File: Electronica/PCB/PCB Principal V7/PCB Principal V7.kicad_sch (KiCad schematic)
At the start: 18 parts, among them J1 Conexion Sensores, J11 Conn_01x04_Pin, J2 Power Monster, J3 On/Off General, J4 Power Input 2, J5 IDC Placa Botones, J6 Power Input 1, SW1 On/Off Motores, U1 74HC595

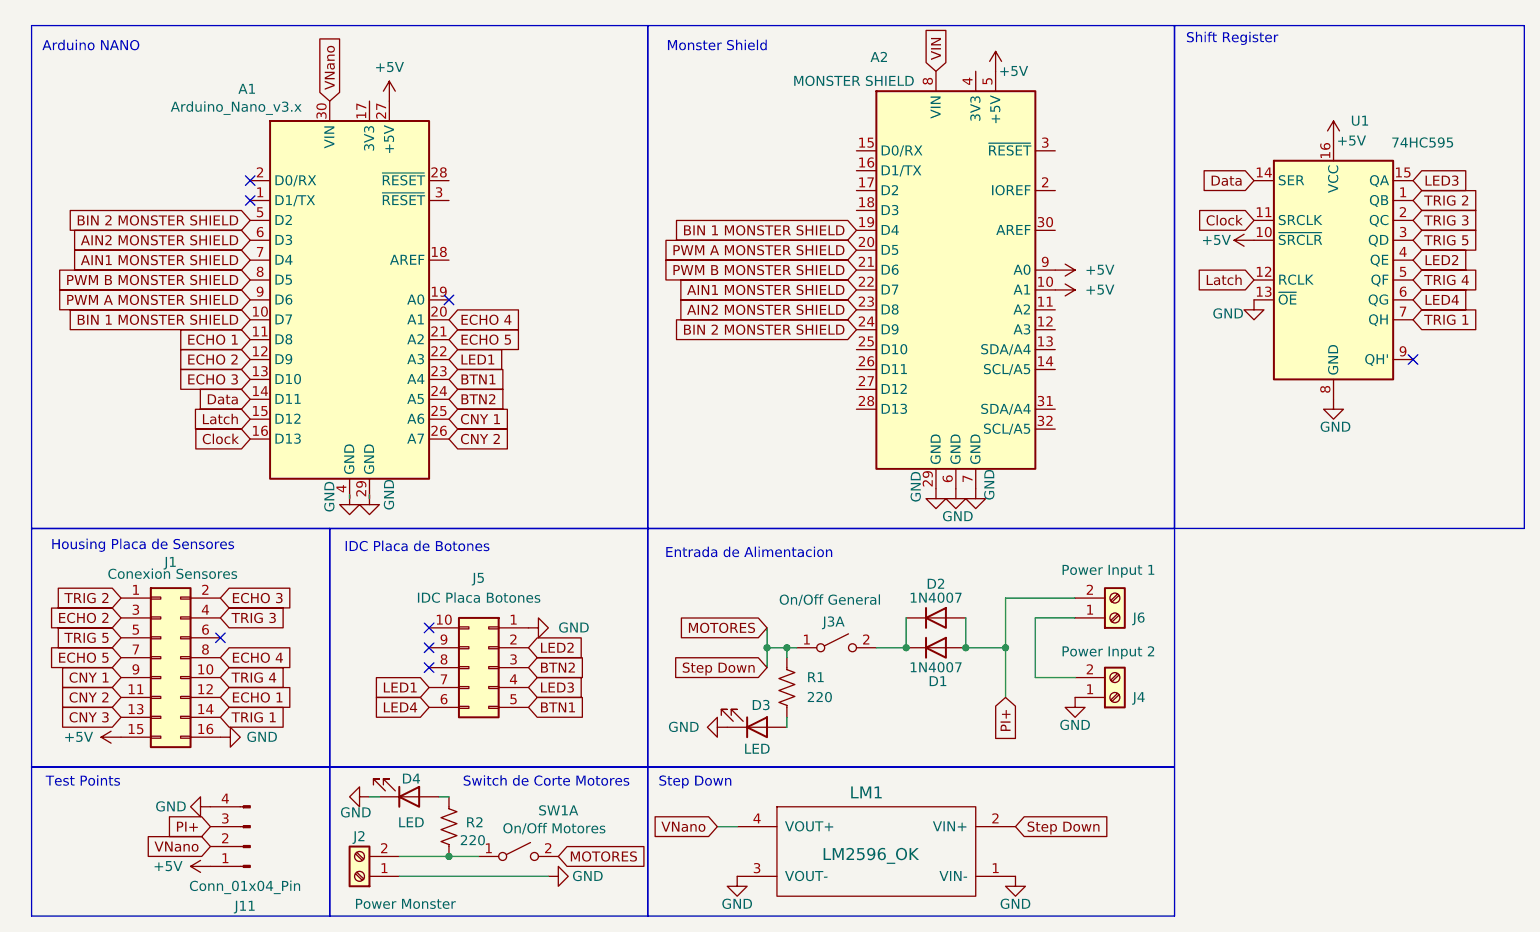
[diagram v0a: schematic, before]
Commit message: PCB sensores v2 y principal v7 terminadas
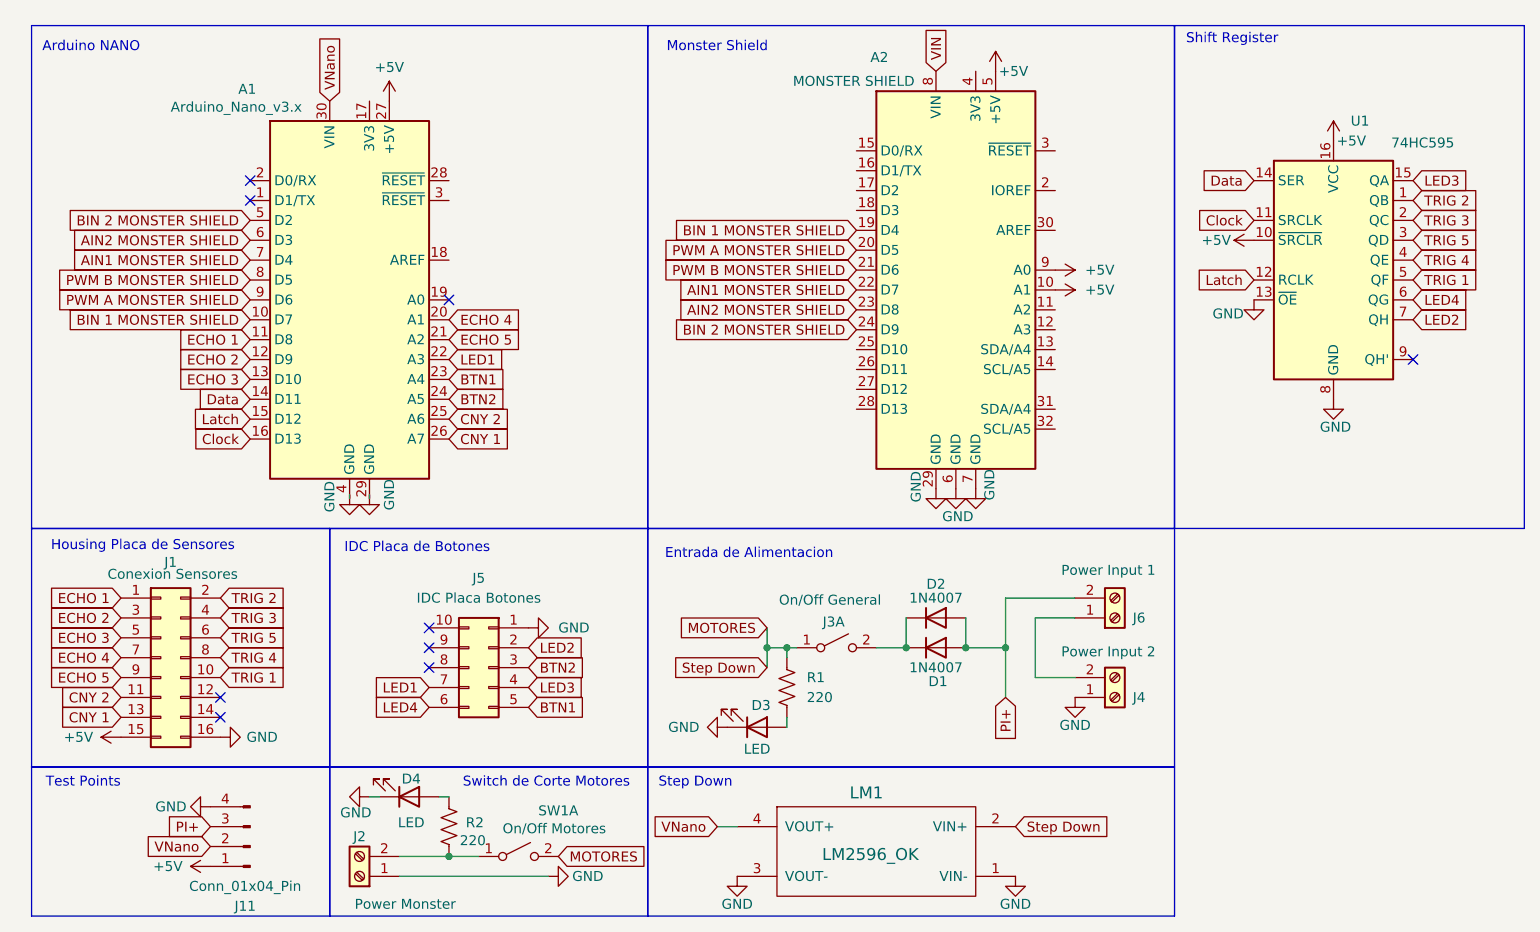
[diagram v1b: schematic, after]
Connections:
- net CNY 3 is gone; now on net CNY 1: J1.13 (Pin_13)
- net CNY 1: now also A1.26 (A7); no longer A1.25 (A6), J1.9 (Pin_9)
- net CNY 2: now also A1.25 (A6); no longer A1.26 (A7)
- net ECHO 1: now also J1.1 (Pin_1); no longer J1.12 (Pin_12)
- net ECHO 3: now also J1.5 (Pin_5); no longer J1.2 (Pin_2)
- net ECHO 4: now also J1.7 (Pin_7); no longer J1.8 (Pin_8)
- net ECHO 5: now also J1.9 (Pin_9); no longer J1.7 (Pin_7)
- net LED2: now also U1.7 (QH); no longer U1.4 (QE)
- net TRIG 1: now also J1.10 (Pin_10), U1.5 (QF); no longer J1.14 (Pin_14), U1.7 (QH)
- net TRIG 2: now also J1.2 (Pin_2); no longer J1.1 (Pin_1)
- net TRIG 4: now also J1.8 (Pin_8), U1.4 (QE); no longer J1.10 (Pin_10), U1.5 (QF)
- net TRIG 5: now also J1.6 (Pin_6); no longer J1.5 (Pin_5)
- no-connect marks 8 -> 9
